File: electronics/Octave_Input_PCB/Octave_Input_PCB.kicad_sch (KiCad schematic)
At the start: 57 parts, among them J1 HRO_TYPE-C-31-M-12, SW1 SW_Hot_Swap_Socket, SW10 SW_Hot_Swap_Socket, SW11 SW_Hot_Swap_Socket, SW12 SW_Hot_Swap_Socket, SW13 SW_Hot_Swap_Socket, SW14 Alps_Alpine_RKJXV1224, SW15 Bourns_PEC12R-4xxxF-Sxxx, SW2 SW_Hot_Swap_Socket, SW3 SW_Hot_Swap_Socket, SW4 SW_Hot_Swap_Socket, SW5 SW_Hot_Swap_Socket, SW6 SW_Hot_Swap_Socket, SW7 SW_Hot_Swap_Socket, SW8 SW_Hot_Swap_Socket, SW9 SW_Hot_Swap_Socket, U1 AP2112K-3.3, U2 Raspberry_Pi_RP2040

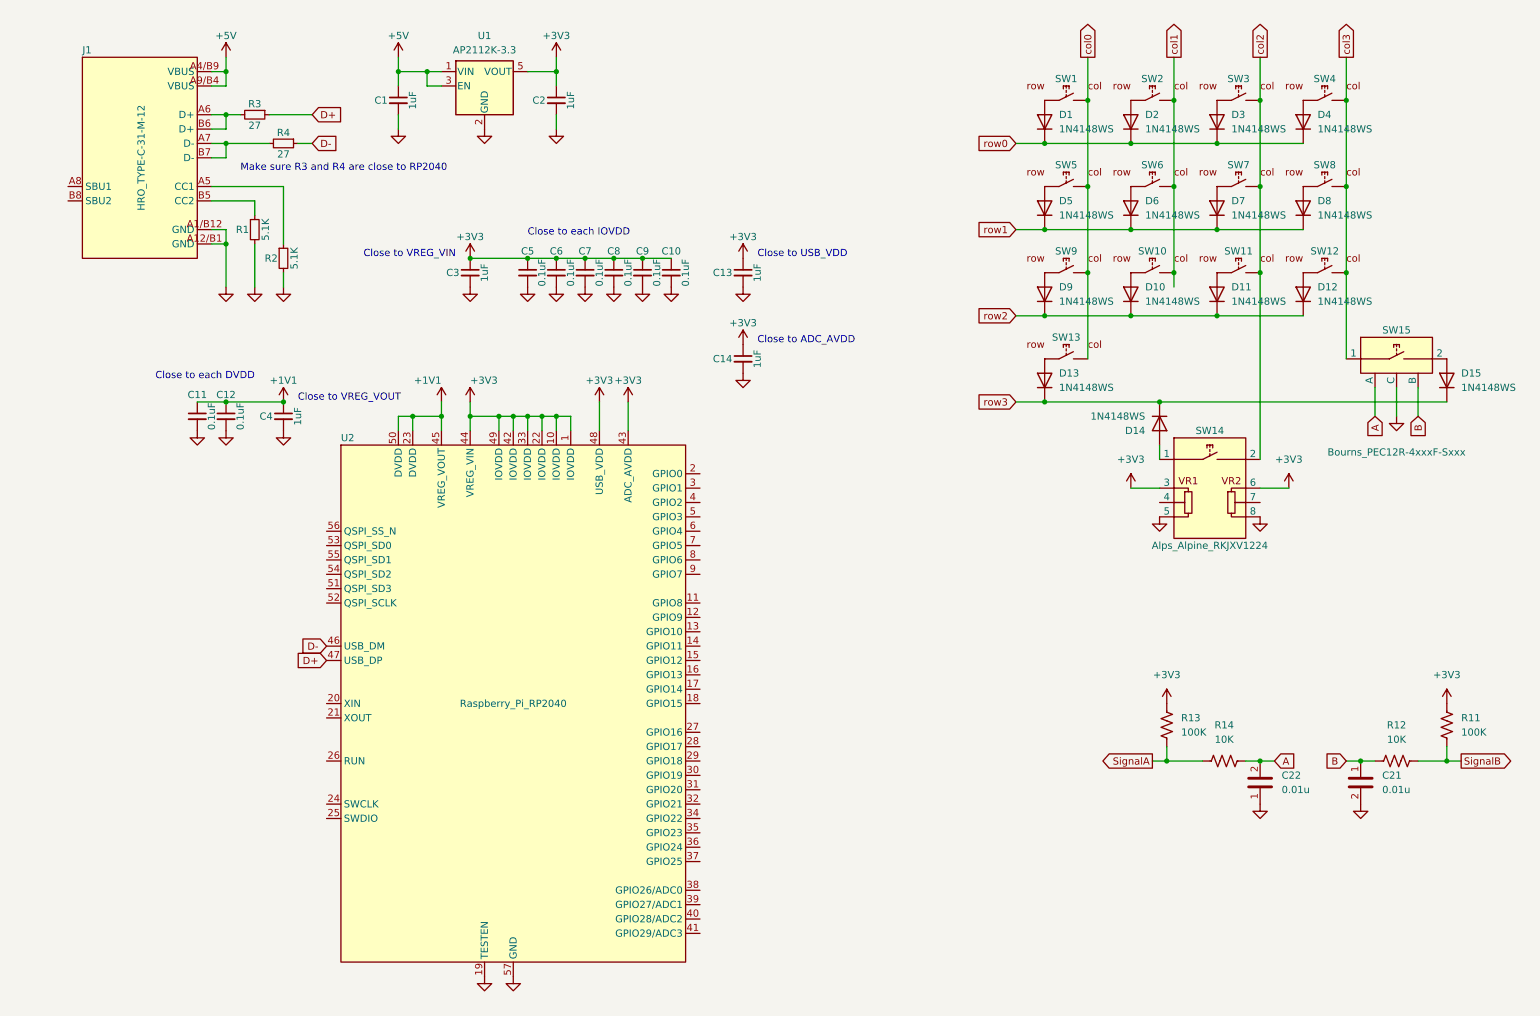
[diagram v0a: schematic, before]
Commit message: [WIP] Update schematic and PCB
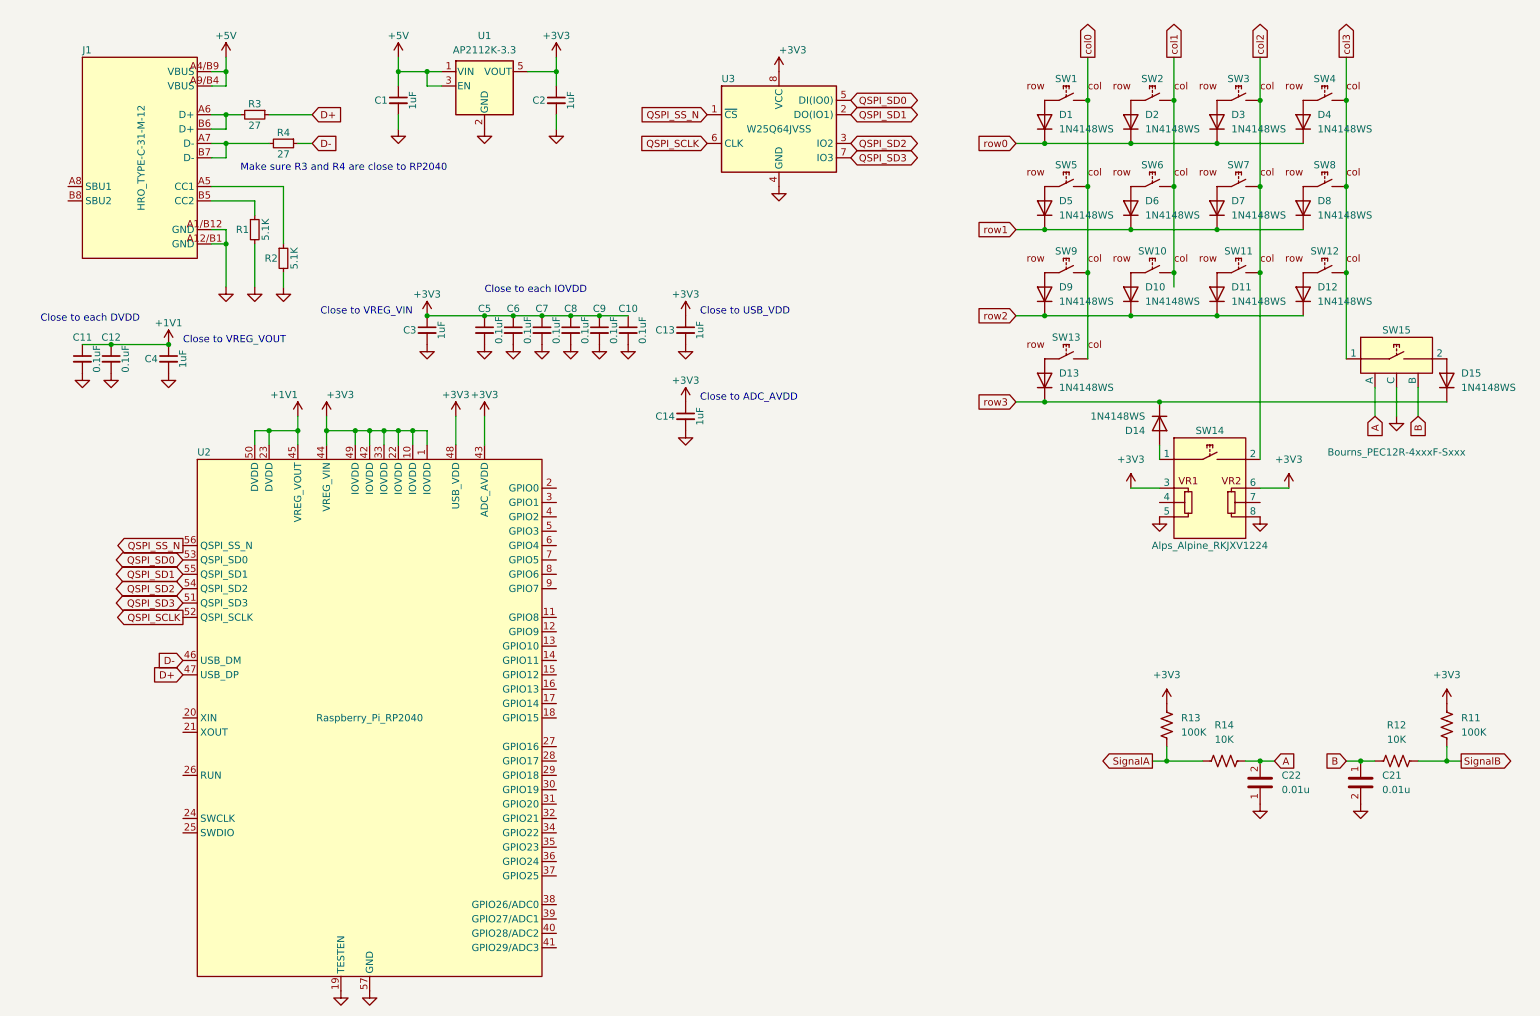
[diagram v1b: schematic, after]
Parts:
- added U3: W25Q64JVSS, Package_SO:SOIC-8_5.23x5.23mm_P1.27mm, symbol Memory_Flash:W25Q32JVSS
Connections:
- net +3V3: now also U3.8 (VCC)
- net GND: now also U3.4 (GND)
- net QSPI_SD3: now reaches U2.51 (QSPI_SD3)
- net QSPI_SD3: now also U3.7 (IO3)
- net QSPI_SCLK: now reaches U2.52 (QSPI_SCLK)
- net QSPI_SCLK: now also U3.6 (CLK)
- net QSPI_SD0: now reaches U2.53 (QSPI_SD0)
- net QSPI_SD0: now also U3.5 (DI(IO0))
- net QSPI_SD2: now reaches U2.54 (QSPI_SD2)
- net QSPI_SD2: now also U3.3 (IO2)
- net QSPI_SD1: now reaches U2.55 (QSPI_SD1)
- net QSPI_SD1: now also U3.2 (DO(IO1))
- net QSPI_SS_N: now reaches U2.56 (QSPI_SS_N)
- net QSPI_SS_N: now also U3.1 (~{CS})
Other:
- moved on the sheet: C10, C11, C12, C13, C14, C3, C4, C5, C6, C7, C8, C9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
